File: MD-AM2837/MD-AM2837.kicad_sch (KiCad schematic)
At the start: 13 parts, among them J1 XT60_Male_Horizontal, J2 XT60_Female_Horizontal, J3 Conn_01x03_Pin_signal

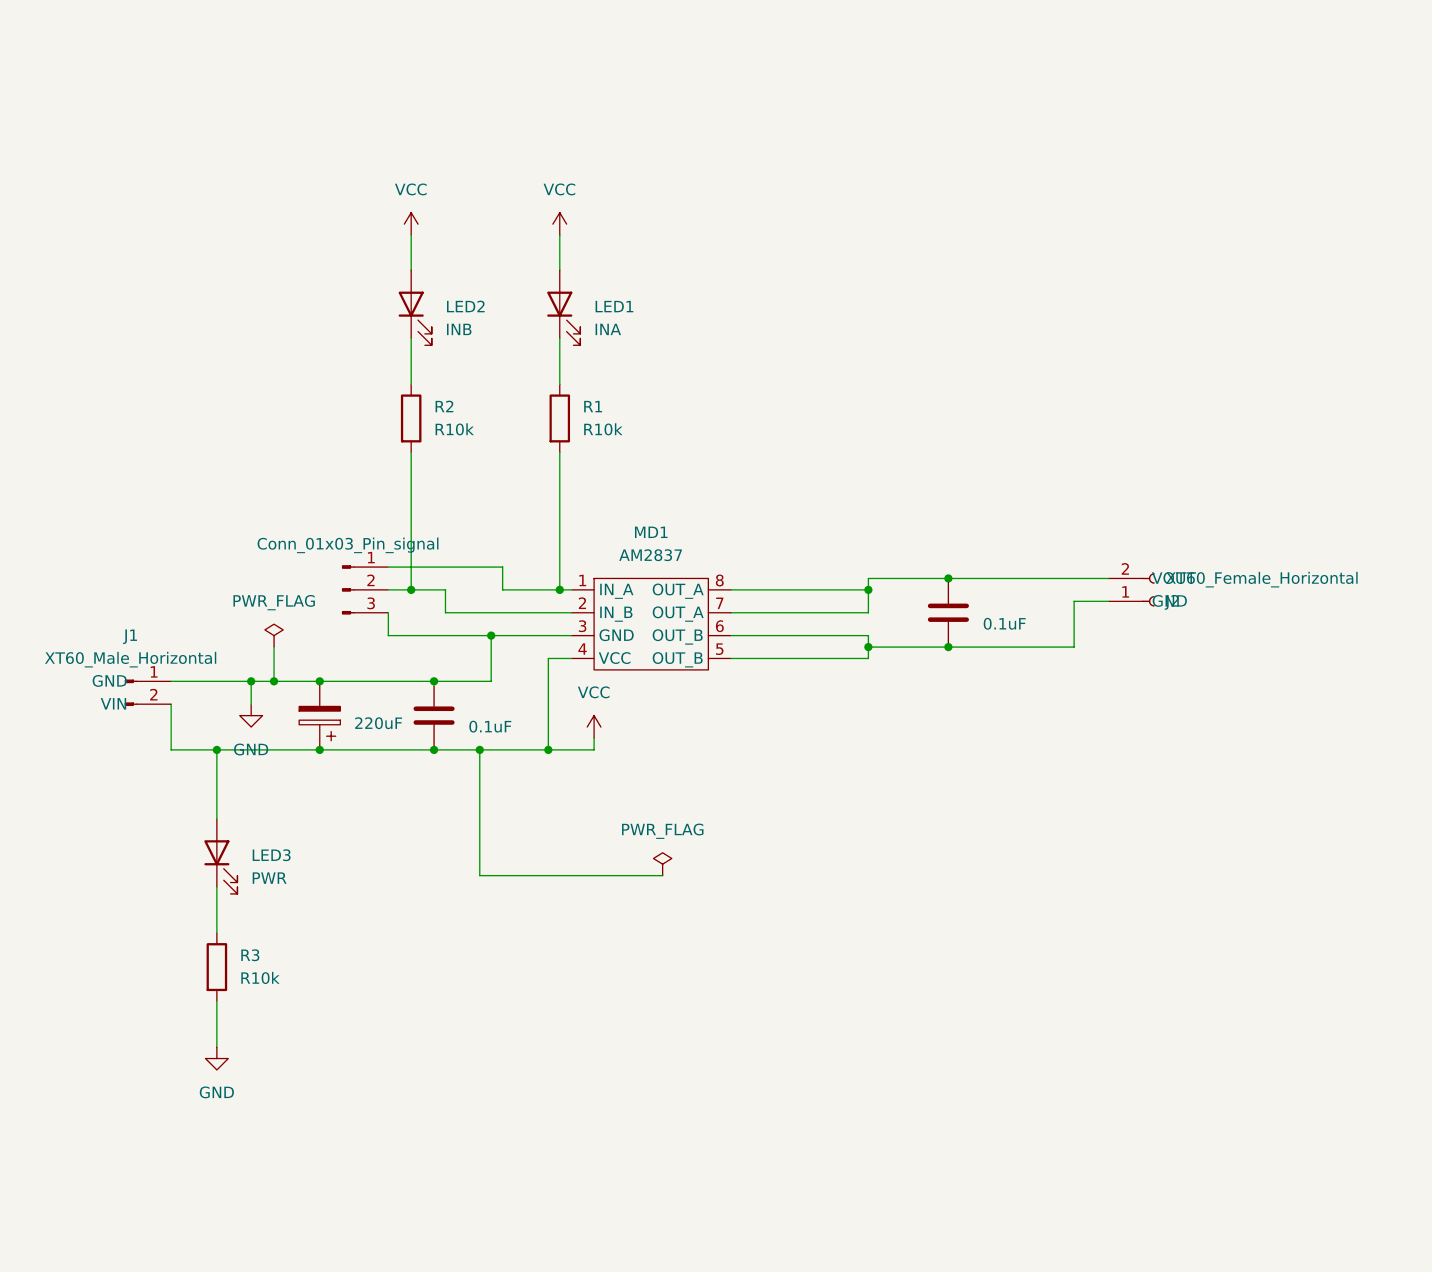
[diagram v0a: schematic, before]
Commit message: v0.1
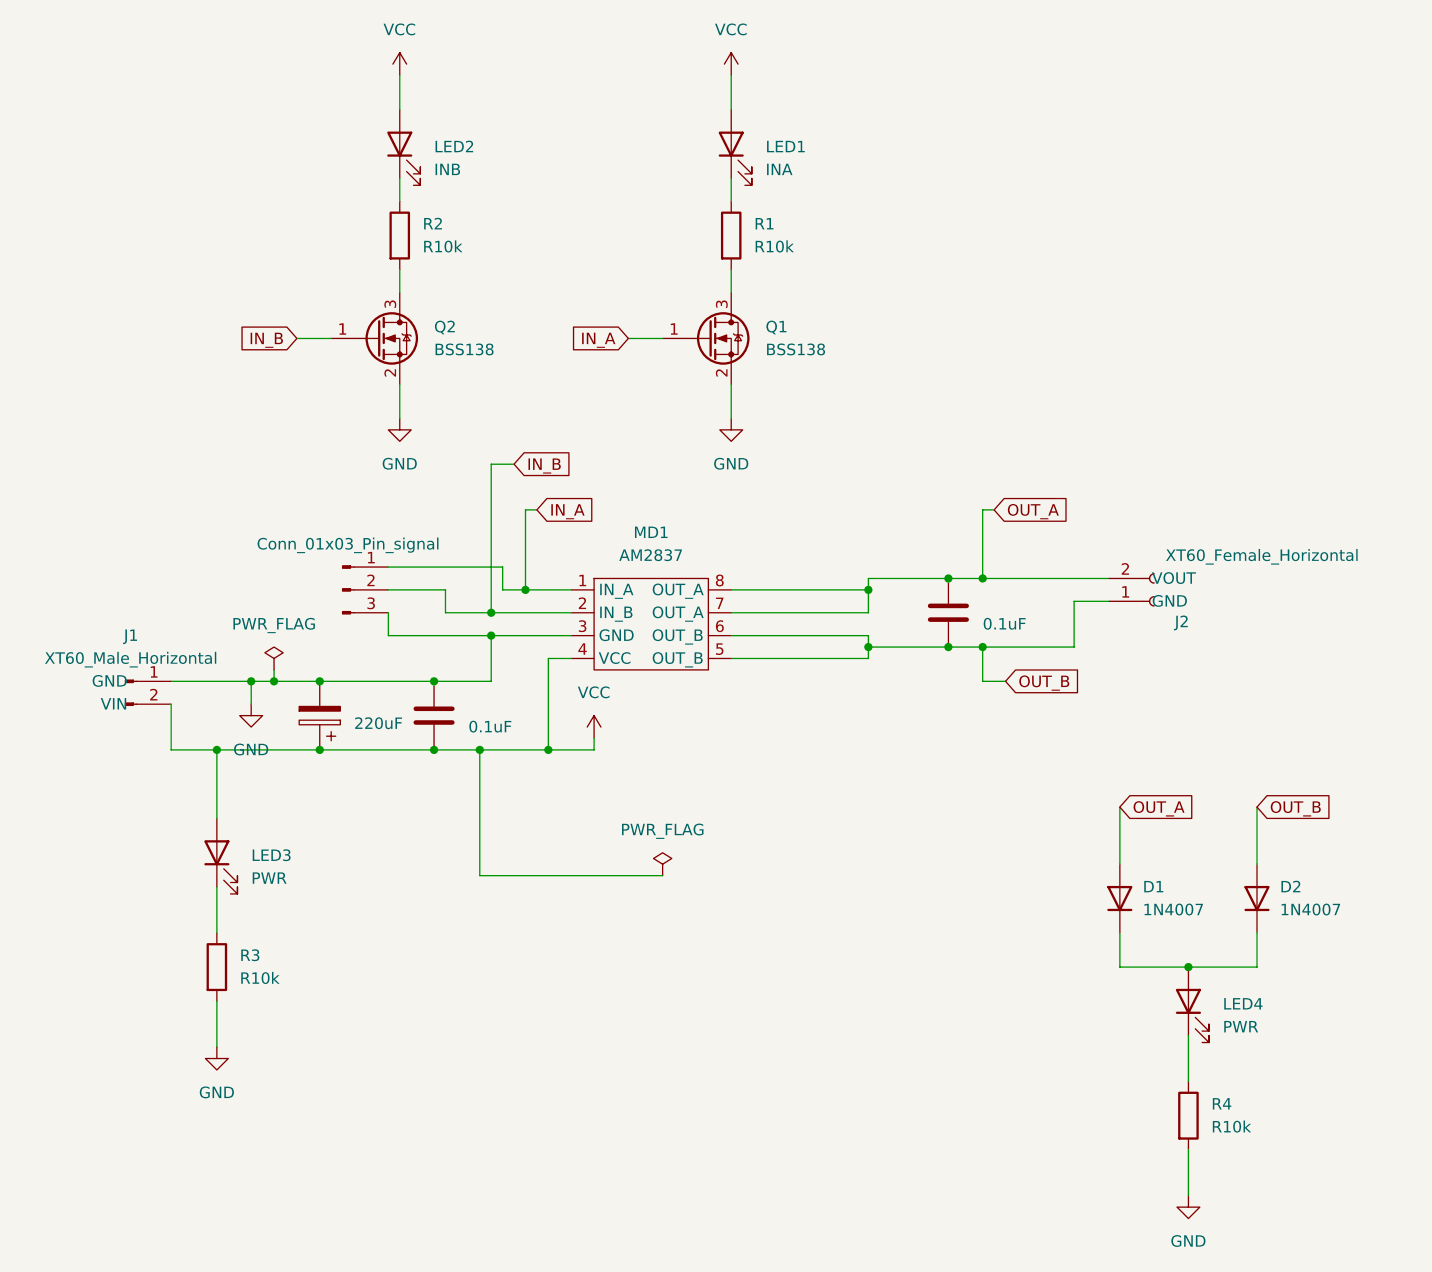
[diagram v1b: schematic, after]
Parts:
- added D1, D2: 1N4007, Diode_THT:D_DO-41_SOD81_P10.16mm_Horizontal, symbol Diode:1N4007
- added LED4: PWR, LED_SMD:LED_0603_1608Metric_Pad1.05x0.95mm_HandSolder, symbol 00_mylib:LED1608
- added Q1, Q2: BSS138, Package_TO_SOT_SMD:SOT-23, symbol Transistor_FET:BSS138
- added R4: R10k, Resistor_SMD:R_0603_1608Metric_Pad0.98x0.95mm_HandSolder, symbol 00_mylib:R1608
- C1: footprint Capacitor_SMD:C_Elec_10x10.2 -> Capacitor_THT:C_Radial_D8.0mm_H11.5mm_P3.50mm
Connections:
- net GND: now also Q1.2 (S), Q2.2 (S), R4.2
- net IN_A: now reaches J3.1 (Pin_1), MD1.1 (IN_A)
- net IN_A: now also Q1.1 (G); no longer R1.2
- net IN_B: now reaches J3.2 (Pin_2), MD1.2 (IN_B)
- net IN_B: now also Q2.1 (G); no longer R2.2
- net OUT_A: now reaches C3.1, J2.2 (VOUT), MD1.7 (OUT_A), MD1.8 (OUT_A)
- net OUT_A: now also D1.2 (A)
- net OUT_B: now reaches C3.2, J2.1 (GND), MD1.5 (OUT_B), MD1.6 (OUT_B)
- net OUT_B: now also D2.2 (A)
- new net: Q2.3 (D), R2.2
- new net: D1.1 (K), D2.1 (K), LED4.2 (A)
- new net: LED4.1 (K), R4.1
- new net: Q1.3 (D), R1.2
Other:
- moved on the sheet: LED1, LED2, R1, R2
